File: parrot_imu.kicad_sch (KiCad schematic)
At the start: 6 parts

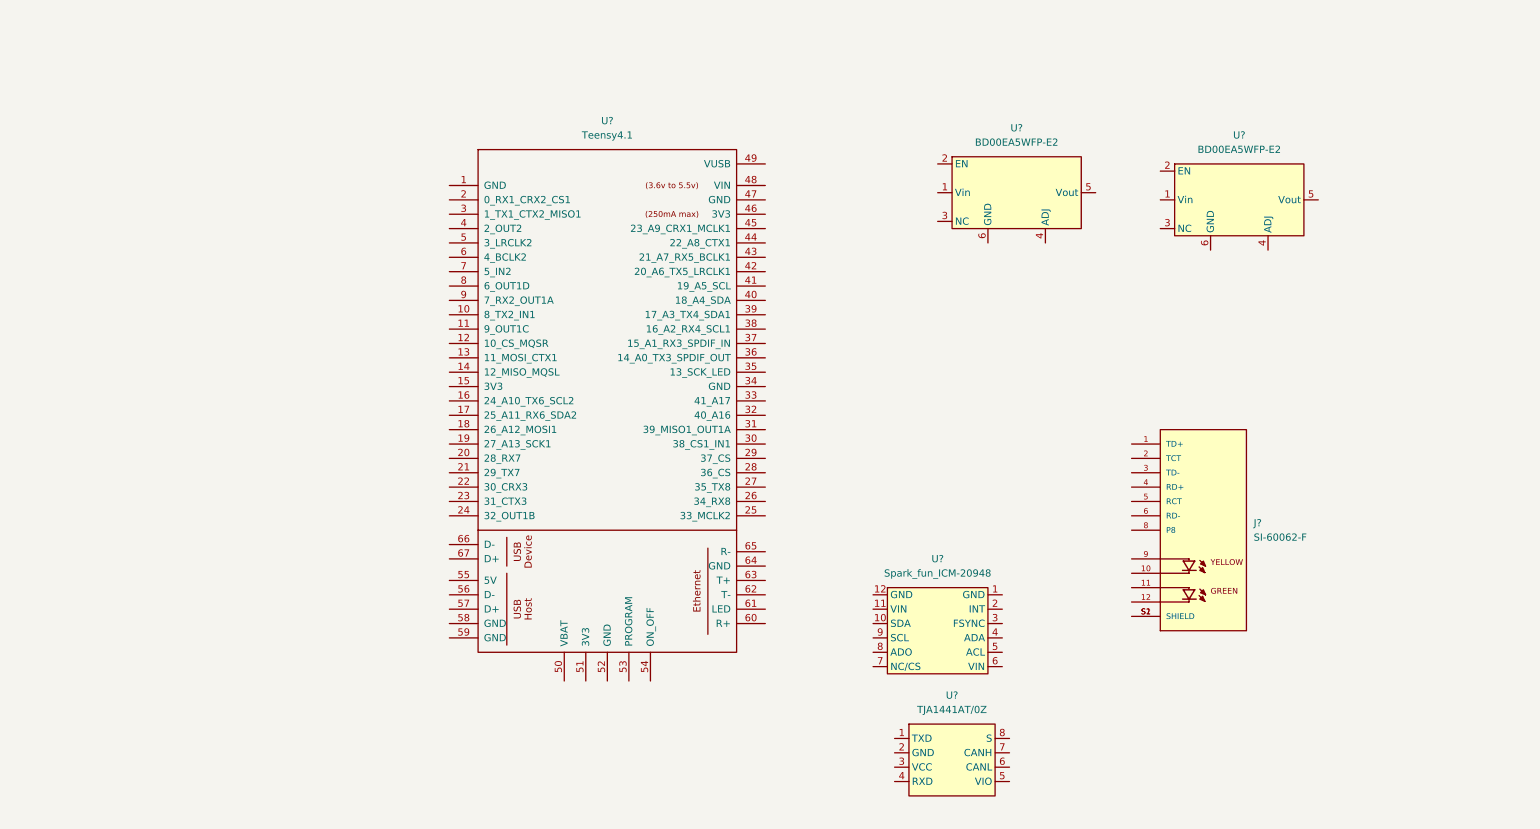
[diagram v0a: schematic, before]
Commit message: some progress on the schematic and notes on other things to handle
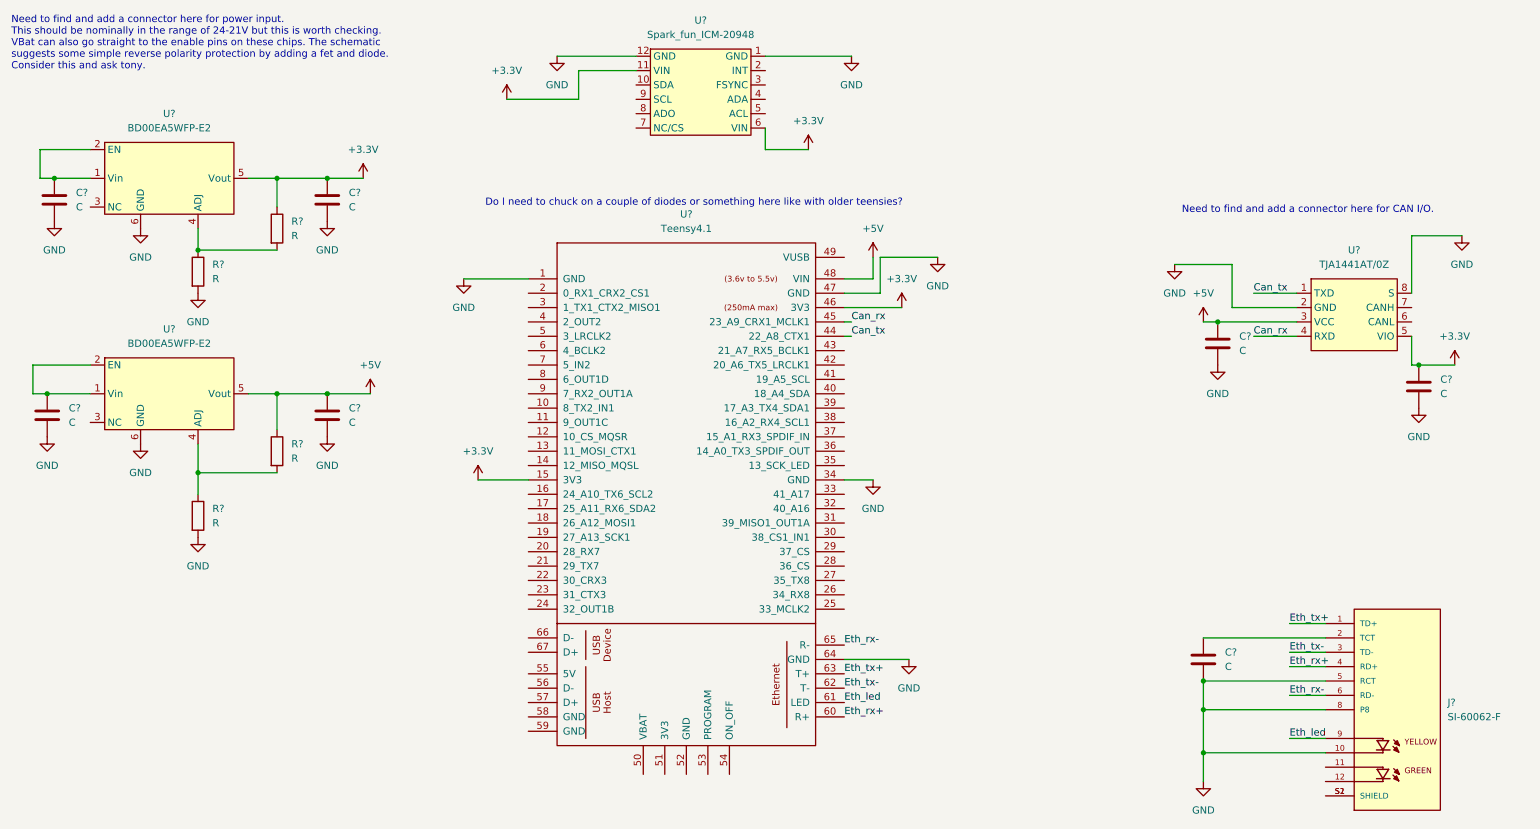
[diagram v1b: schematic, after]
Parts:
- added C? (x7): C, symbol Device:C
- added R? (x4): R, symbol Device:R
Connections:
- net at U?.1 (Vin): now also U?.2 (EN), C?.1 (x2)
- net at U?.4 (ADJ): now also R?.1, R?.2 (x2)
- net +5V: now reaches U?.5 (Vout)
- net +5V: now also U?.3 (VCC), U?.48 (VIN), C?.1, C?.1, R?.1
- net GND: now reaches U?.6 (GND)
- net GND: now also J?.10, J?.5 (RCT), J?.8 (P8), U?.1 (GND), U?.1 (GND), U?.12 (GND), U?.2 (GND), U?.34 (GND), U?.47 (GND), U?.6 (GND), U?.64 (GND), U?.8 (S), C?.2, C?.2, C?.2, C?.2, C?.2, C?.2, C?.2, R?.2, R?.2
- net Can_tx: now reaches U?.1 (TXD)
- net Can_tx: now also U?.44 (22_A8_CTX1)
- net Can_rx: now reaches U?.4 (RXD)
- net Can_rx: now also U?.45 (23_A9_CRX1_MCLK1)
- net +3.3V: now reaches U?.5 (VIO)
- net +3.3V: now also U?.11 (VIN), U?.15 (3V3), U?.46 (3V3), U?.5 (Vout), U?.6 (VIN), C?.1, C?.1, R?.1
- net Eth_rx+: now reaches U?.60 (R+)
- net Eth_rx+: now also J?.4 (RD+)
- net Eth_led: now reaches U?.61 (LED)
- net Eth_led: now also J?.9
- net Eth_tx-: now reaches U?.62 (T-)
- net Eth_tx-: now also J?.3 (TD-)
- net Eth_tx+: now reaches U?.63 (T+)
- net Eth_tx+: now also J?.1 (TD+)
- net Eth_rx-: now reaches U?.65 (R-)
- net Eth_rx-: now also J?.6 (RD-)
- net at J?.2 (TCT): now also C?.1
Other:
- note added: "Do I need to chuck on a couple of diodes or something here like with older teensies?"
- note added: "Need to find and add a connector here for CAN I/O."
- note added: "Need to find and add a connector here for power input. This should be nominally in the range of 24-21V but this is worth checking. VBat can also go straight to the enable pins on these chips. The schematic suggests some simple reverse polarity protection by adding a fet and diode. Consider this and ask tony."
- moved on the sheet: J?, U?
